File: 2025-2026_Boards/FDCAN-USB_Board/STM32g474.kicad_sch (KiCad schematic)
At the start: 12 parts, among them J4 Conn_01x02_Pin, J5 Conn_01x02_Pin, J6 Conn_ARM_JTAG_SWD_10, U3 STM32G474CETx

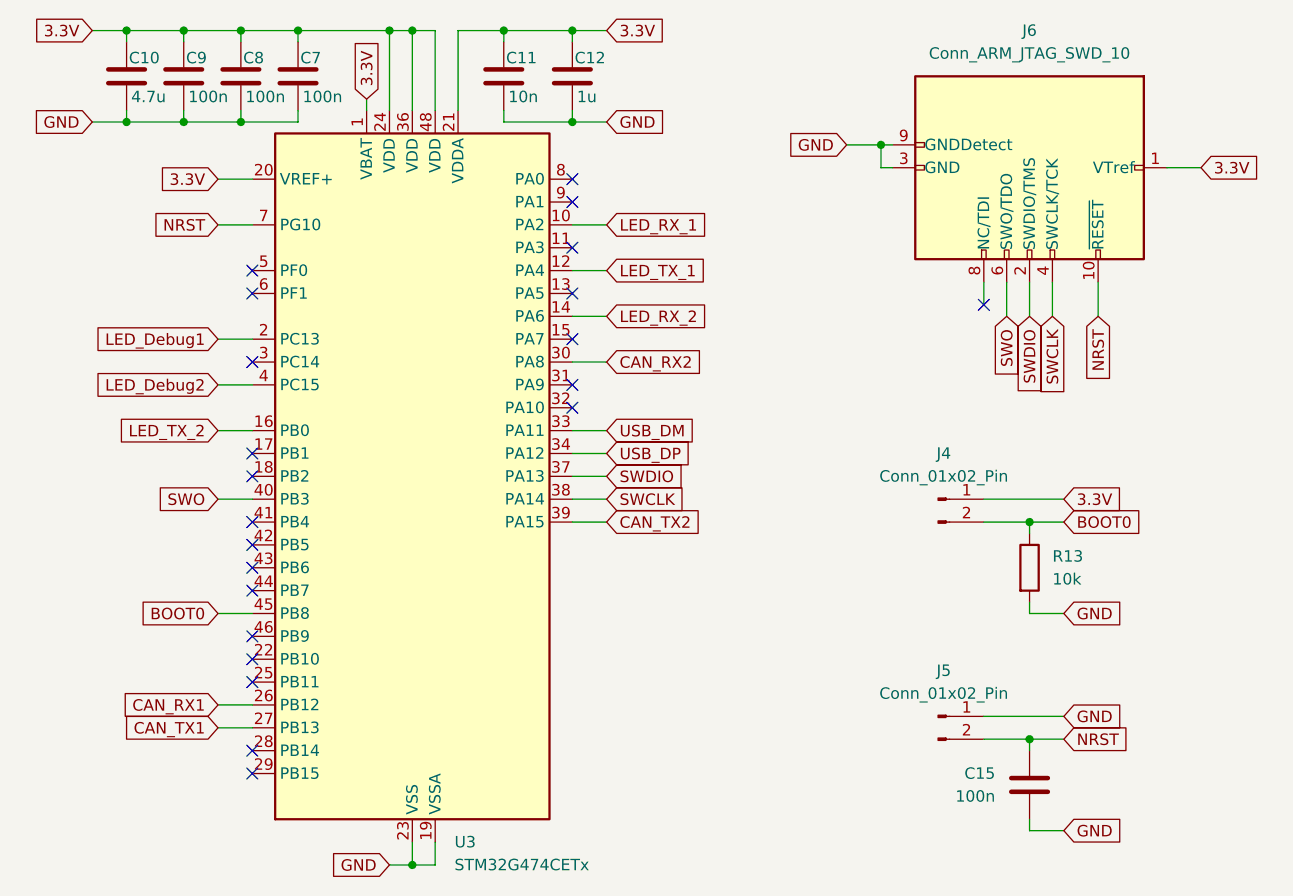
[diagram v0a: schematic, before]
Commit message: Layout finished
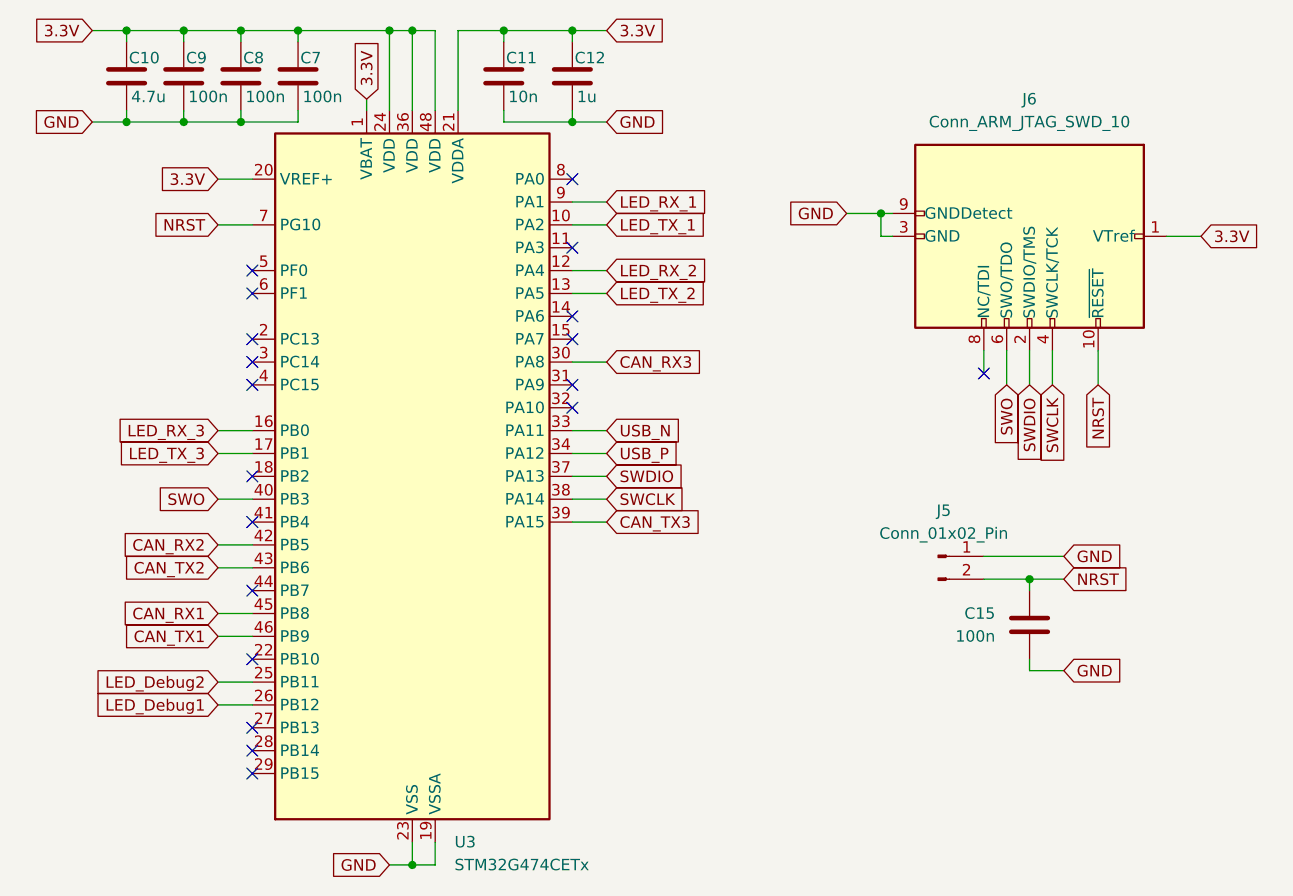
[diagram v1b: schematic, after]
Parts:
- removed J4: Conn_01x02_Pin, Connector_PinHeader_2.54mm:PinHeader_1x02_P2.54mm_Vertical, symbol Connector:Conn_01x02_Pin
- removed R13: 10k, Resistor_SMD:R_0603_1608Metric, symbol Device:R
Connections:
- net BOOT0 is gone; now on net CAN_RX1: U3.45 (PB8)
- net CAN_RX1: no longer U3.26 (PB12)
- net CAN_RX2: now also U3.42 (PB5); no longer U3.30 (PA8)
- net CAN_TX1: now also U3.46 (PB9); no longer U3.27 (PB13)
- net CAN_TX2: now also U3.43 (PB6); no longer U3.39 (PA15)
- net LED_Debug1: now also U3.26 (PB12); no longer U3.2 (PC13)
- net LED_Debug2: now also U3.25 (PB11); no longer U3.4 (PC15)
- net LED_RX_1: now also U3.9 (PA1); no longer U3.10 (PA2)
- net LED_RX_2: now also U3.12 (PA4); no longer U3.14 (PA6)
- net LED_TX_1: now also U3.10 (PA2); no longer U3.12 (PA4)
- net LED_TX_2: now also U3.13 (PA5); no longer U3.16 (PB0)
- net LED_TX_3: now reaches U3.17 (PB1)
- net USB_DM renamed USB_N
- net USB_DP renamed USB_P
- new net CAN_RX3: U3.30 (PA8)
- new net CAN_TX3: U3.39 (PA15)
- new net LED_RX_3: U3.16 (PB0)
- no-connect marks 22 -> 19
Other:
- moved on the sheet: C15, J5, J6
